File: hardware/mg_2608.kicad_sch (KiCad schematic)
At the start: 27 parts, among them IC1 DALC208SC6, J1 JAE_SIM_Card_SF72S006

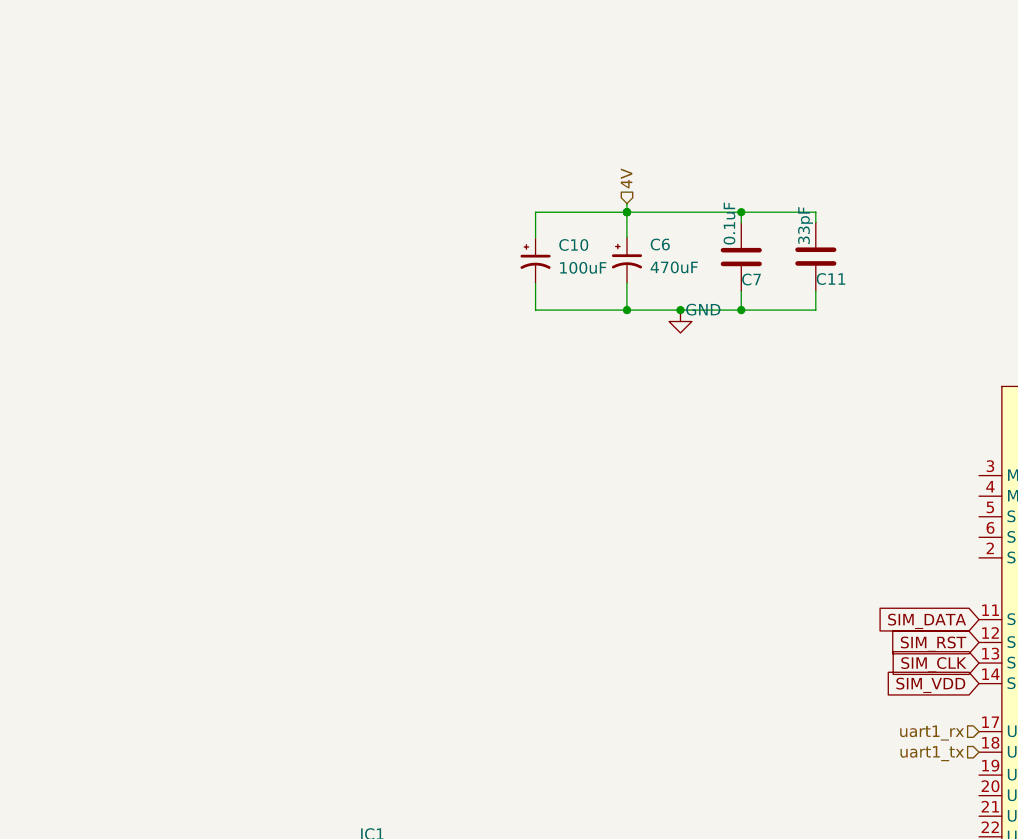
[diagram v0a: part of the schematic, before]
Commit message: Kicad düzenleme.
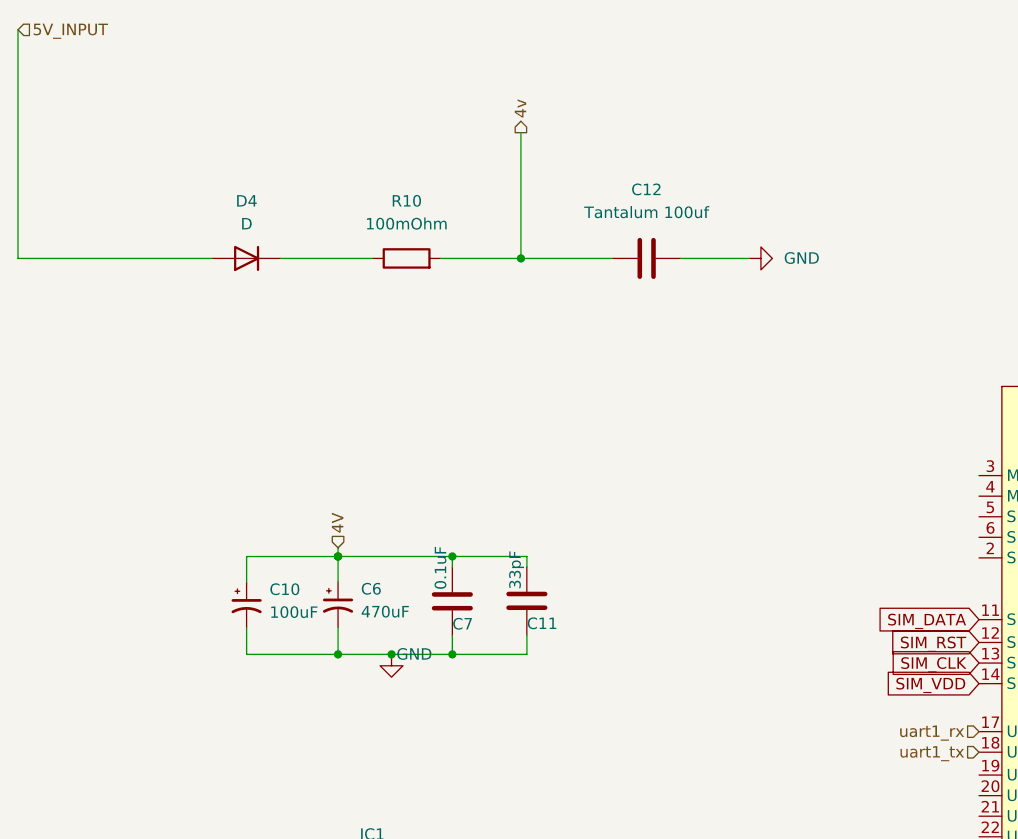
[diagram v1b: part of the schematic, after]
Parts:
- added C12: Tantalum 100uf, symbol Device:C
- added D4: D, symbol Device:D
- added R10: 100mOhm, symbol Device:R
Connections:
- net GND: now also C12.2
- new net: D4.1 (K), R10.1
- new net 4v: C12.1, R10.2
- new net 5V_INPUT: D4.2 (A)
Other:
- moved on the sheet: C10, C11, C6, C7
